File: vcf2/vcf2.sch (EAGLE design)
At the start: 115 parts, among them IC1 OPA4130U, IC2 OPA4130U, IC3 OPA4130U, IC4 OPA4130U, IC5 OPA4130U, Q7 BC847ASMD

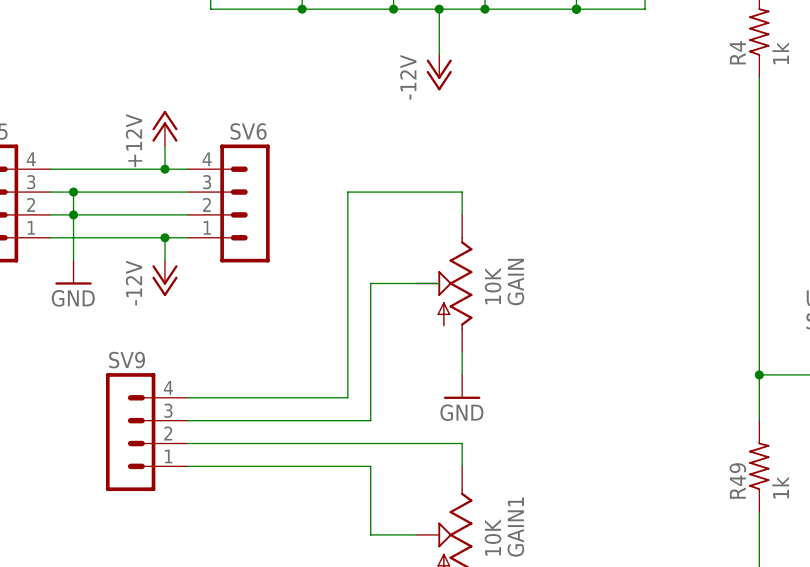
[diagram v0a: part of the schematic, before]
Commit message: made gerbers for vcf2
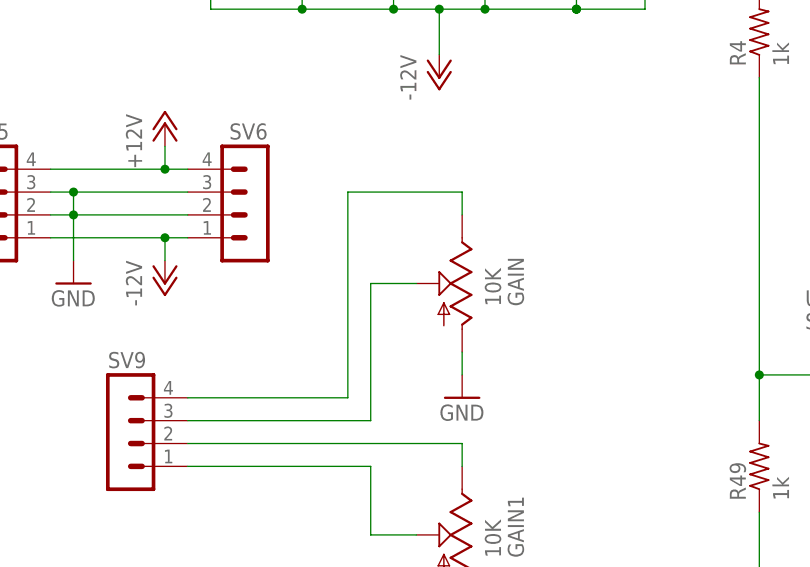
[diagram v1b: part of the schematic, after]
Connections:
- net N$86: now also GAIN.S
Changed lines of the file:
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@@
 <wire x1="-43.18" y1="81.28" x2="-22.86" y2="81.28" width="0.1524" layer="91"/>
 <wire x1="-22.86" y1="81.28" x2="-22.86" y2="96.52" width="0.1524" layer="91"/>
-<wire x1="-22.86" y1="96.52" x2="-15.24" y2="96.52" width="0.1524" layer="91"/>
+<wire x1="-22.86" y1="96.52" x2="-17.78" y2="96.52" width="0.1524" layer="91"/>
+<pinref part="GAIN" gate="G$1" pin="S"/>
 </segment>
 </net>
